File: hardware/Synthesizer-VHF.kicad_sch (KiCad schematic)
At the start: 93 parts, among them J1 Screw_Terminal_01x02, J2 Scope, J4 USB-C 2.0 16P, J5 REF_IN, J6 Scope, J7 RFOUTA, J8 Header 1x3, J9 RFOUTB, U1 LM7805A, U2 FT231XQ, U3 ATtiny1616-M, U4 ADF4351, U5 USBLC6-2SC6, U7 ADP150AUJZ-3.3-R7, U8 ADP150AUJZ-3.3-R7, X1 HCI 8122S-25NQ33FTL

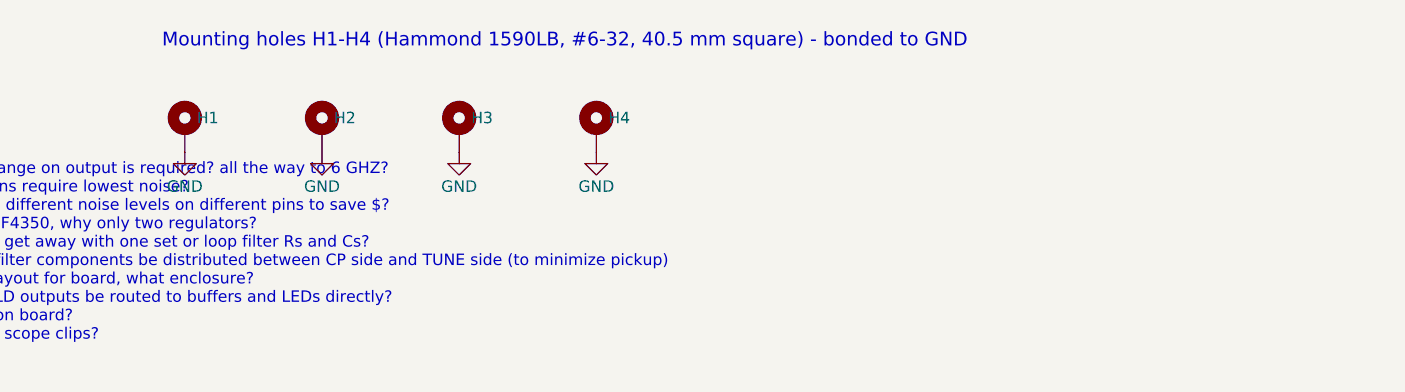
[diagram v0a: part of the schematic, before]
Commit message: diecast-2x2: user layout edits (KiCad save)
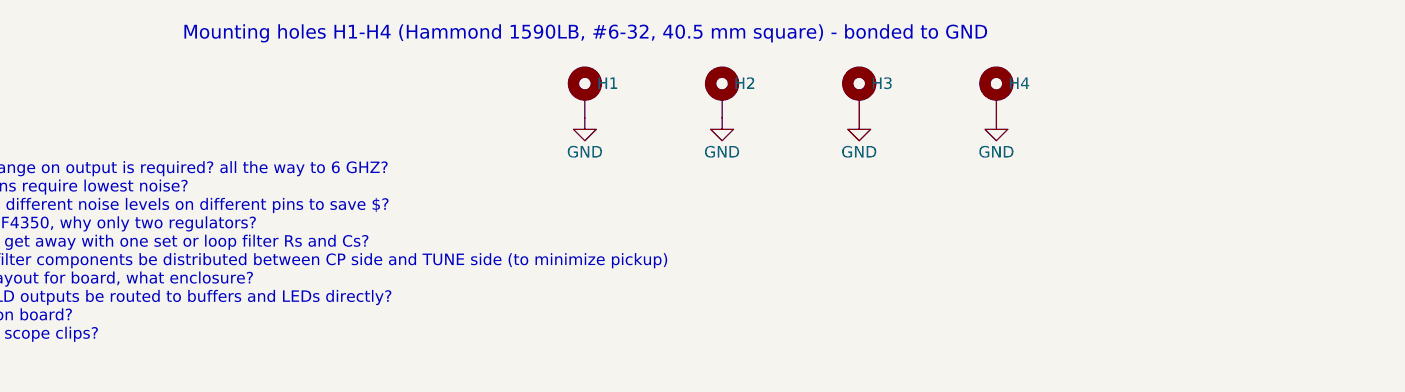
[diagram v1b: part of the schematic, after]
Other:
- moved on the sheet: H1, H2, H3, H4
